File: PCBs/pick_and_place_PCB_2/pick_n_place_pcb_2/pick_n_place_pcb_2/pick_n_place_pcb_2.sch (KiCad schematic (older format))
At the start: 8 parts, among them J1 Conn_01x04, J2 Conn_01x04, U1 Pick_and_place_pcb, U2 24AA02-OT

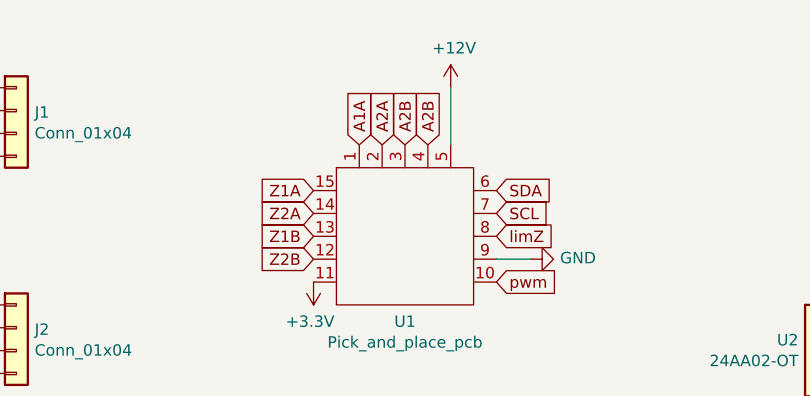
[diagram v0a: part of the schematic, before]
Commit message: modify kicad and freecad
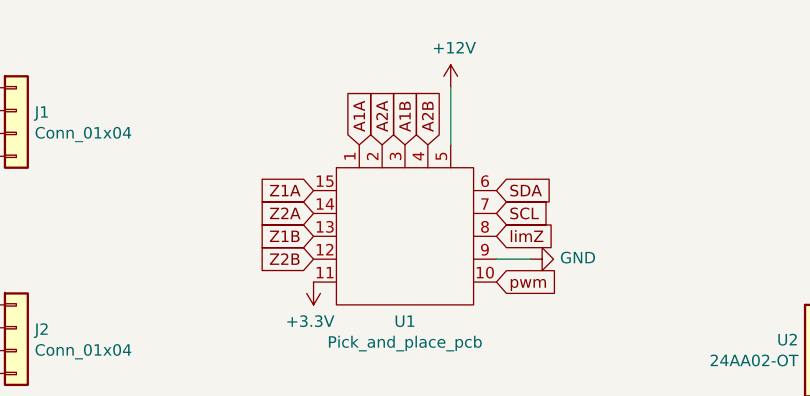
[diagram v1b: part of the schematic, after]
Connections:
- net A1B: now also U1.3
- net A2B: no longer U1.3
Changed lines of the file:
@@
 A2A
 Text GLabel 5750 3300 1    50   Input ~ 0
-A2B
+A1B
 Text GLabel 5850 3300 1    50   Input ~ 0
 A2B
